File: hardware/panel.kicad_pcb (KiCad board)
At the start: 2 copper layers, 99.2 x 100 mm, 1073 parts, among them J1 USB_A_Embedded, U1 CH32V203F8U6, U2 XC6206PxxxMR

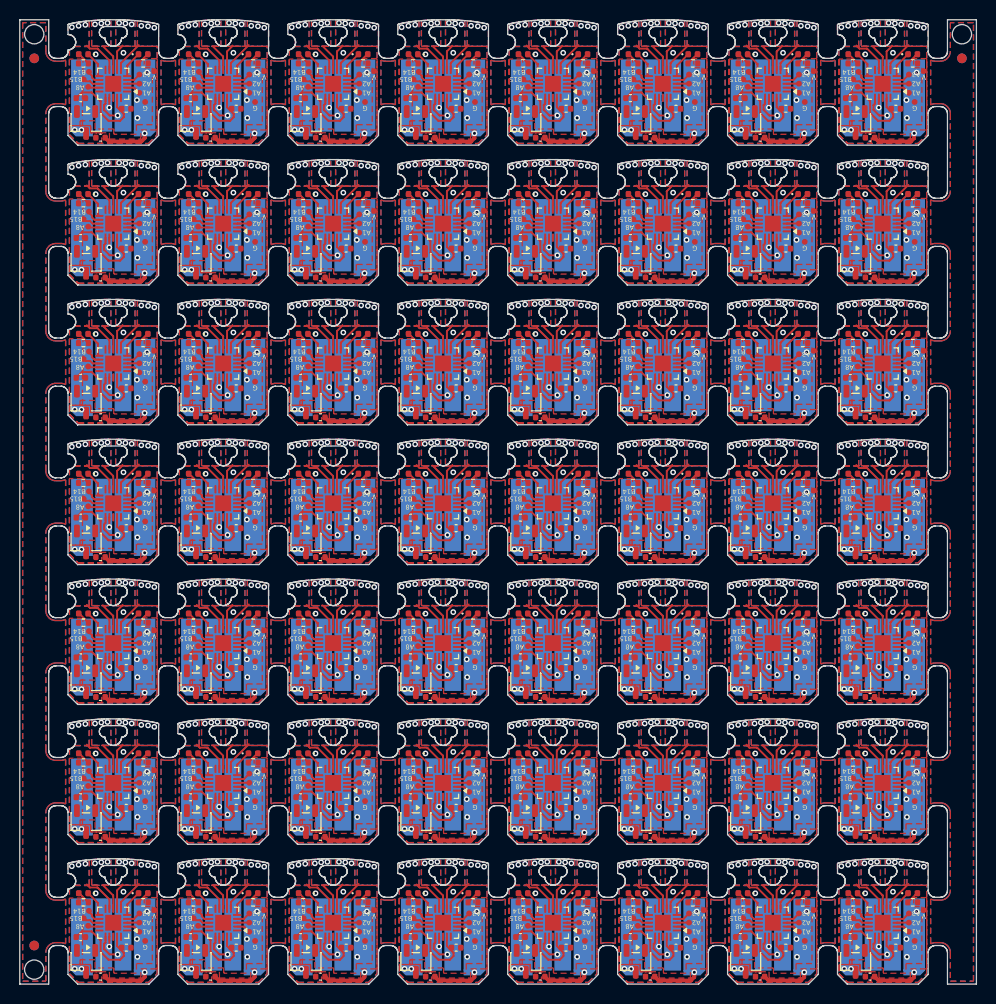
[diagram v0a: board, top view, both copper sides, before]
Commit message: Update
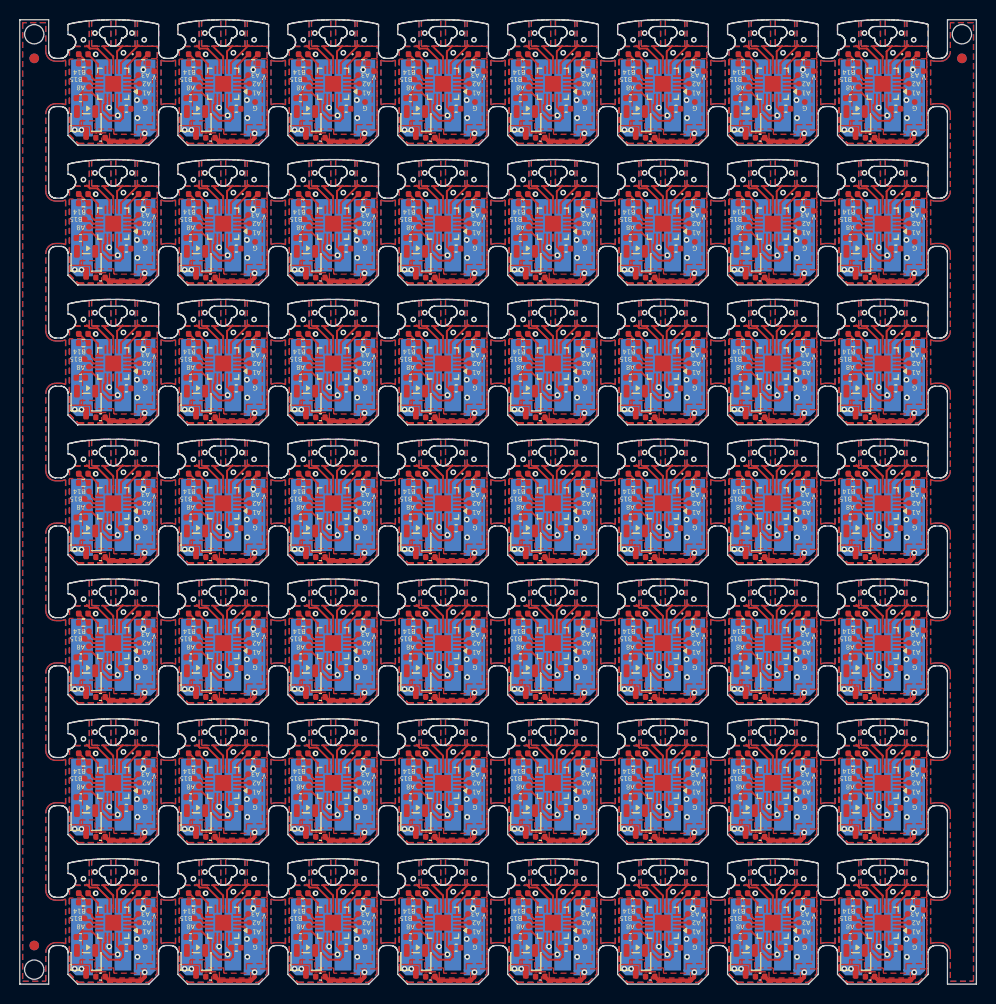
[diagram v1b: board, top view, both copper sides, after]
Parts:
- removed the TP1 at (145.5, 112.7)
- removed the TP1 at (134.1, 25.7)
- removed the TP1 at (156.9, 83.7)
- removed the TP1 at (168.3, 98.2)
- removed the TP1 at (156.9, 54.7)
- removed the TP1 at (122.7, 54.7)
- removed the TP1 at (145.5, 54.7)
- removed the TP1 at (111.3, 83.7)
- removed the TP1 at (122.7, 69.2)
- removed the TP1 at (122.7, 112.7)
- removed the TP1 at (145.5, 98.2)
- removed the TP1 at (156.9, 25.7)
- removed the TP1 at (122.7, 40.2)
- removed the TP1 at (145.5, 40.2)
- removed the TP1 at (111.3, 112.7)
- removed the TP1 at (179.7, 25.7)
- removed the TP1 at (191.1, 112.7)
- removed the TP1 at (179.7, 112.7)
- removed the TP1 at (191.1, 98.2)
- removed the TP1 at (168.3, 25.7)
- removed the TP1 at (134.1, 69.2)
- removed the TP1 at (111.3, 54.7)
- removed the TP1 at (111.3, 40.2)
- removed the TP1 at (145.5, 83.7)
- removed the TP1 at (111.3, 25.7)
- removed the TP1 at (134.1, 40.2)
- removed the TP1 at (111.3, 69.2)
- removed the TP1 at (145.5, 25.7)
- removed the TP1 at (134.1, 83.7)
- removed the TP1 at (156.9, 69.2)
- removed the TP1 at (168.3, 54.7)
- removed the TP1 at (168.3, 112.7)
- removed the TP1 at (122.7, 83.7)
- removed the TP1 at (179.7, 69.2)
- removed the TP1 at (168.3, 69.2)
- removed the TP1 at (134.1, 112.7)
- removed the TP1 at (191.1, 25.7)
- removed the TP1 at (156.9, 112.7)
- removed the TP1 at (111.3, 98.2)
- removed the TP1 at (145.5, 69.2)
- removed the TP1 at (179.7, 98.2)
- removed the TP1 at (179.7, 54.7)
- removed the TP1 at (191.1, 69.2)
- removed the TP1 at (156.9, 98.2)
- removed the TP1 at (156.9, 40.2)
- removed the TP1 at (134.1, 98.2)
- removed the TP1 at (191.1, 83.7)
- removed the TP1 at (134.1, 54.7)
- removed the TP1 at (168.3, 83.7)
- removed the TP1 at (122.7, 98.2)
- removed the TP1 at (122.7, 25.7)
- removed the TP1 at (179.7, 40.2)
- removed the TP1 at (168.3, 40.2)
- removed the TP1 at (179.7, 83.7)
- removed the TP1 at (191.1, 54.7)
- removed the TP1 at (191.1, 40.2)
- removed the TP5 at (185.3, 55.2)
- removed the TP5 at (105.5, 69.7)
- removed the TP5 at (151.1, 98.7)
- removed the TP5 at (185.3, 113.2)
- removed the TP5 at (139.7, 26.2)
- removed the TP5 at (173.9, 84.2)
- removed the TP5 at (173.9, 69.7)
- removed the TP5 at (128.3, 84.2)
- removed the TP5 at (139.7, 98.7)
- removed the TP5 at (105.5, 55.2)
- removed the TP5 at (185.3, 98.7)
- removed the TP5 at (185.3, 69.7)
- removed the TP5 at (116.9, 98.7)
- removed the TP5 at (162.5, 113.2)
- removed the TP5 at (151.1, 55.2)
- removed the TP5 at (128.3, 69.7)
- removed the TP5 at (151.1, 113.2)
- removed the TP5 at (185.3, 26.2)
- removed the TP5 at (139.7, 40.7)
- removed the TP5 at (116.9, 84.2)
- removed the TP5 at (162.5, 55.2)
- removed the TP5 at (128.3, 40.7)
- removed the TP5 at (173.9, 40.7)
- removed the TP5 at (139.7, 69.7)
- removed the TP5 at (128.3, 113.2)
- removed the TP5 at (105.5, 84.2)
- removed the TP5 at (116.9, 26.2)
- removed the TP5 at (139.7, 55.2)
- removed the TP5 at (105.5, 113.2)
- removed the TP5 at (151.1, 26.2)
- removed the TP5 at (139.7, 113.2)
- removed the TP5 at (105.5, 98.7)
- removed the TP5 at (162.5, 40.7)
- removed the TP5 at (128.3, 26.2)
- removed the TP5 at (173.9, 55.2)
- removed the TP5 at (116.9, 113.2)
- removed the TP5 at (173.9, 26.2)
- removed the TP5 at (105.5, 26.2)
- removed the TP5 at (185.3, 84.2)
- removed the TP5 at (185.3, 40.7)
- removed the TP5 at (162.5, 84.2)
- removed the TP5 at (162.5, 26.2)
- removed the TP5 at (173.9, 98.7)
- removed the TP5 at (105.5, 40.7)
- removed the TP5 at (151.1, 40.7)
- removed the TP5 at (116.9, 40.7)
- removed the TP5 at (151.1, 84.2)
- removed the TP5 at (173.9, 113.2)
- removed the TP5 at (116.9, 69.7)
- removed the TP5 at (151.1, 69.7)
- removed the TP5 at (162.5, 98.7)
- removed the TP5 at (128.3, 55.2)
- removed the TP5 at (128.3, 98.7)
- removed the TP5 at (139.7, 84.2)
- removed the TP5 at (162.5, 69.7)
- removed the TP5 at (116.9, 55.2)
- removed the TP6 at (106.0, 56.0)
- removed the TP6 at (140.2, 70.5)
- removed the TP6 at (140.2, 114.0)
- removed the TP6 at (106.0, 85.0)
- removed the TP6 at (140.2, 56.0)
- removed the TP6 at (151.6, 41.5)
- removed the TP6 at (117.4, 70.5)
- removed the TP6 at (117.4, 56.0)
- removed the TP6 at (106.0, 41.5)
- removed the TP6 at (163.0, 85.0)
- removed the TP6 at (106.0, 70.5)
- removed the TP6 at (163.0, 114.0)
- removed the TP6 at (117.4, 85.0)
- removed the TP6 at (185.8, 85.0)
- removed the TP6 at (185.8, 70.5)
- removed the TP6 at (151.6, 99.5)
- removed the TP6 at (185.8, 41.5)
- removed the TP6 at (140.2, 99.5)
- removed the TP6 at (185.8, 114.0)
- removed the TP6 at (163.0, 70.5)
- removed the TP6 at (174.4, 114.0)
- removed the TP6 at (128.8, 41.5)
- removed the TP6 at (106.0, 114.0)
- removed the TP6 at (151.6, 56.0)
- removed the TP6 at (174.4, 41.5)
- removed the TP6 at (174.4, 56.0)
- removed the TP6 at (140.2, 27.0)
- removed the TP6 at (174.4, 85.0)
- removed the TP6 at (128.8, 99.5)
- removed the TP6 at (117.4, 41.5)
- removed the TP6 at (151.6, 85.0)
- removed the TP6 at (163.0, 27.0)
- removed the TP6 at (128.8, 56.0)
- removed the TP6 at (117.4, 114.0)
- removed the TP6 at (185.8, 56.0)
- removed the TP6 at (151.6, 114.0)
- removed the TP6 at (117.4, 27.0)
- removed the TP6 at (128.8, 27.0)
- removed the TP6 at (117.4, 99.5)
- removed the TP6 at (128.8, 70.5)
- removed the TP6 at (106.0, 27.0)
- removed the TP6 at (128.8, 85.0)
- removed the TP6 at (163.0, 41.5)
- removed the TP6 at (106.0, 99.5)
- removed the TP6 at (174.4, 99.5)
- removed the TP6 at (163.0, 56.0)
- removed the TP6 at (151.6, 70.5)
- removed the TP6 at (163.0, 99.5)
- removed the TP6 at (151.6, 27.0)
- removed the TP6 at (128.8, 114.0)
- removed the TP6 at (185.8, 27.0)
- removed the TP6 at (174.4, 70.5)
- removed the TP6 at (140.2, 41.5)
- removed the TP6 at (140.2, 85.0)
- removed the TP6 at (174.4, 27.0)
- removed the TP6 at (185.8, 99.5)
- added TP1: TestPoint, ch32:TestPoint_Pad_D0.6mm, F.Cu at (168.2, 83.7)
- added TP1: TestPoint, ch32:TestPoint_Pad_D0.6mm, F.Cu at (156.8, 69.2)
- added TP1: TestPoint, ch32:TestPoint_Pad_D0.6mm, F.Cu at (145.4, 40.2)
- added TP1: TestPoint, ch32:TestPoint_Pad_D0.6mm, F.Cu at (179.6, 69.2)
- added TP1: TestPoint, ch32:TestPoint_Pad_D0.6mm, F.Cu at (179.6, 112.7)
- added TP1: TestPoint, ch32:TestPoint_Pad_D0.6mm, F.Cu at (111.2, 69.2)
- added TP1: TestPoint, ch32:TestPoint_Pad_D0.6mm, F.Cu at (111.2, 83.7)
- added TP1: TestPoint, ch32:TestPoint_Pad_D0.6mm, F.Cu at (179.6, 83.7)
- added TP1: TestPoint, ch32:TestPoint_Pad_D0.6mm, F.Cu at (122.6, 25.7)
- added TP1: TestPoint, ch32:TestPoint_Pad_D0.6mm, F.Cu at (156.8, 54.7)
- added TP1: TestPoint, ch32:TestPoint_Pad_D0.6mm, F.Cu at (134.0, 40.2)
- added TP1: TestPoint, ch32:TestPoint_Pad_D0.6mm, F.Cu at (168.2, 54.7)
- added TP1: TestPoint, ch32:TestPoint_Pad_D0.6mm, F.Cu at (134.0, 25.7)
- added TP1: TestPoint, ch32:TestPoint_Pad_D0.6mm, F.Cu at (156.8, 83.7)
- added TP1: TestPoint, ch32:TestPoint_Pad_D0.6mm, F.Cu at (156.8, 98.2)
- added TP1: TestPoint, ch32:TestPoint_Pad_D0.6mm, F.Cu at (191.0, 69.2)
- added TP1: TestPoint, ch32:TestPoint_Pad_D0.6mm, F.Cu at (134.0, 83.7)
- added TP1: TestPoint, ch32:TestPoint_Pad_D0.6mm, F.Cu at (134.0, 112.7)
- added TP1: TestPoint, ch32:TestPoint_Pad_D0.6mm, F.Cu at (111.2, 54.7)
- added TP1: TestPoint, ch32:TestPoint_Pad_D0.6mm, F.Cu at (145.4, 98.2)
- added TP1: TestPoint, ch32:TestPoint_Pad_D0.6mm, F.Cu at (134.0, 69.2)
- added TP1: TestPoint, ch32:TestPoint_Pad_D0.6mm, F.Cu at (168.2, 112.7)
- added TP1: TestPoint, ch32:TestPoint_Pad_D0.6mm, F.Cu at (111.2, 40.2)
- added TP1: TestPoint, ch32:TestPoint_Pad_D0.6mm, F.Cu at (179.6, 25.7)
- added TP1: TestPoint, ch32:TestPoint_Pad_D0.6mm, F.Cu at (145.4, 25.7)
- added TP1: TestPoint, ch32:TestPoint_Pad_D0.6mm, F.Cu at (134.0, 54.7)
- added TP1: TestPoint, ch32:TestPoint_Pad_D0.6mm, F.Cu at (111.2, 25.7)
- added TP1: TestPoint, ch32:TestPoint_Pad_D0.6mm, F.Cu at (191.0, 112.7)
- added TP1: TestPoint, ch32:TestPoint_Pad_D0.6mm, F.Cu at (191.0, 83.7)
- added TP1: TestPoint, ch32:TestPoint_Pad_D0.6mm, F.Cu at (191.0, 25.7)
- added TP1: TestPoint, ch32:TestPoint_Pad_D0.6mm, F.Cu at (122.6, 40.2)
- added TP1: TestPoint, ch32:TestPoint_Pad_D0.6mm, F.Cu at (111.2, 98.2)
- added TP1: TestPoint, ch32:TestPoint_Pad_D0.6mm, F.Cu at (122.6, 83.7)
- added TP1: TestPoint, ch32:TestPoint_Pad_D0.6mm, F.Cu at (168.2, 69.2)
- added TP1: TestPoint, ch32:TestPoint_Pad_D0.6mm, F.Cu at (145.4, 54.7)
- added TP1: TestPoint, ch32:TestPoint_Pad_D0.6mm, F.Cu at (145.4, 112.7)
- added TP1: TestPoint, ch32:TestPoint_Pad_D0.6mm, F.Cu at (191.0, 98.2)
- added TP1: TestPoint, ch32:TestPoint_Pad_D0.6mm, F.Cu at (179.6, 40.2)
- added TP1: TestPoint, ch32:TestPoint_Pad_D0.6mm, F.Cu at (168.2, 25.7)
- added TP1: TestPoint, ch32:TestPoint_Pad_D0.6mm, F.Cu at (122.6, 54.7)
- added TP1: TestPoint, ch32:TestPoint_Pad_D0.6mm, F.Cu at (145.4, 83.7)
- added TP1: TestPoint, ch32:TestPoint_Pad_D0.6mm, F.Cu at (122.6, 98.2)
- added TP1: TestPoint, ch32:TestPoint_Pad_D0.6mm, F.Cu at (156.8, 40.2)
- added TP1: TestPoint, ch32:TestPoint_Pad_D0.6mm, F.Cu at (156.8, 112.7)
- added TP1: TestPoint, ch32:TestPoint_Pad_D0.6mm, F.Cu at (168.2, 98.2)
- added TP1: TestPoint, ch32:TestPoint_Pad_D0.6mm, F.Cu at (179.6, 98.2)
- added TP1: TestPoint, ch32:TestPoint_Pad_D0.6mm, F.Cu at (111.2, 112.7)
- added TP1: TestPoint, ch32:TestPoint_Pad_D0.6mm, F.Cu at (122.6, 69.2)
- added TP1: TestPoint, ch32:TestPoint_Pad_D0.6mm, F.Cu at (168.2, 40.2)
- added TP1: TestPoint, ch32:TestPoint_Pad_D0.6mm, F.Cu at (191.0, 54.7)
- added TP1: TestPoint, ch32:TestPoint_Pad_D0.6mm, F.Cu at (134.0, 98.2)
- added TP1: TestPoint, ch32:TestPoint_Pad_D0.6mm, F.Cu at (145.4, 69.2)
- added TP1: TestPoint, ch32:TestPoint_Pad_D0.6mm, F.Cu at (191.0, 40.2)
- added TP1: TestPoint, ch32:TestPoint_Pad_D0.6mm, F.Cu at (122.6, 112.7)
- added TP1: TestPoint, ch32:TestPoint_Pad_D0.6mm, F.Cu at (179.6, 54.7)
- added TP1: TestPoint, ch32:TestPoint_Pad_D0.6mm, F.Cu at (156.8, 25.7)
- added TP5: TestPoint, ch32:TestPoint_Pad_D0.6mm, F.Cu at (105.6, 69.7)
- added TP5: TestPoint, ch32:TestPoint_Pad_D0.6mm, F.Cu at (117.0, 69.7)
- added TP5: TestPoint, ch32:TestPoint_Pad_D0.6mm, F.Cu at (174.0, 113.2)
- added TP5: TestPoint, ch32:TestPoint_Pad_D0.6mm, F.Cu at (151.2, 40.7)
- added TP5: TestPoint, ch32:TestPoint_Pad_D0.6mm, F.Cu at (174.0, 98.7)
- added TP5: TestPoint, ch32:TestPoint_Pad_D0.6mm, F.Cu at (162.6, 40.7)
- added TP5: TestPoint, ch32:TestPoint_Pad_D0.6mm, F.Cu at (151.2, 98.7)
- added TP5: TestPoint, ch32:TestPoint_Pad_D0.6mm, F.Cu at (151.2, 69.7)
- added TP5: TestPoint, ch32:TestPoint_Pad_D0.6mm, F.Cu at (185.4, 113.2)
- added TP5: TestPoint, ch32:TestPoint_Pad_D0.6mm, F.Cu at (117.0, 84.2)
- added TP5: TestPoint, ch32:TestPoint_Pad_D0.6mm, F.Cu at (139.8, 26.2)
- added TP5: TestPoint, ch32:TestPoint_Pad_D0.6mm, F.Cu at (139.8, 69.7)
- added TP5: TestPoint, ch32:TestPoint_Pad_D0.6mm, F.Cu at (128.4, 69.7)
- added TP5: TestPoint, ch32:TestPoint_Pad_D0.6mm, F.Cu at (105.6, 98.7)
- added TP5: TestPoint, ch32:TestPoint_Pad_D0.6mm, F.Cu at (162.6, 69.7)
- added TP5: TestPoint, ch32:TestPoint_Pad_D0.6mm, F.Cu at (117.0, 98.7)
- added TP5: TestPoint, ch32:TestPoint_Pad_D0.6mm, F.Cu at (105.6, 113.2)
- added TP5: TestPoint, ch32:TestPoint_Pad_D0.6mm, F.Cu at (174.0, 26.2)
- added TP5: TestPoint, ch32:TestPoint_Pad_D0.6mm, F.Cu at (139.8, 84.2)
- added TP5: TestPoint, ch32:TestPoint_Pad_D0.6mm, F.Cu at (185.4, 55.2)
- added TP5: TestPoint, ch32:TestPoint_Pad_D0.6mm, F.Cu at (128.4, 113.2)
- added TP5: TestPoint, ch32:TestPoint_Pad_D0.6mm, F.Cu at (128.4, 55.2)
- added TP5: TestPoint, ch32:TestPoint_Pad_D0.6mm, F.Cu at (151.2, 84.2)
- added TP5: TestPoint, ch32:TestPoint_Pad_D0.6mm, F.Cu at (185.4, 84.2)
- added TP5: TestPoint, ch32:TestPoint_Pad_D0.6mm, F.Cu at (139.8, 55.2)
- added TP5: TestPoint, ch32:TestPoint_Pad_D0.6mm, F.Cu at (128.4, 84.2)
- added TP5: TestPoint, ch32:TestPoint_Pad_D0.6mm, F.Cu at (105.6, 84.2)
- added TP5: TestPoint, ch32:TestPoint_Pad_D0.6mm, F.Cu at (117.0, 26.2)
- added TP5: TestPoint, ch32:TestPoint_Pad_D0.6mm, F.Cu at (162.6, 98.7)
- added TP5: TestPoint, ch32:TestPoint_Pad_D0.6mm, F.Cu at (185.4, 69.7)
- added TP5: TestPoint, ch32:TestPoint_Pad_D0.6mm, F.Cu at (117.0, 40.7)
- added TP5: TestPoint, ch32:TestPoint_Pad_D0.6mm, F.Cu at (105.6, 55.2)
- added TP5: TestPoint, ch32:TestPoint_Pad_D0.6mm, F.Cu at (185.4, 26.2)
- added TP5: TestPoint, ch32:TestPoint_Pad_D0.6mm, F.Cu at (151.2, 55.2)
- added TP5: TestPoint, ch32:TestPoint_Pad_D0.6mm, F.Cu at (174.0, 69.7)
- added TP5: TestPoint, ch32:TestPoint_Pad_D0.6mm, F.Cu at (151.2, 113.2)
- added TP5: TestPoint, ch32:TestPoint_Pad_D0.6mm, F.Cu at (128.4, 98.7)
- added TP5: TestPoint, ch32:TestPoint_Pad_D0.6mm, F.Cu at (162.6, 84.2)
- added TP5: TestPoint, ch32:TestPoint_Pad_D0.6mm, F.Cu at (162.6, 26.2)
- added TP5: TestPoint, ch32:TestPoint_Pad_D0.6mm, F.Cu at (174.0, 40.7)
- added TP5: TestPoint, ch32:TestPoint_Pad_D0.6mm, F.Cu at (128.4, 26.2)
- added TP5: TestPoint, ch32:TestPoint_Pad_D0.6mm, F.Cu at (185.4, 98.7)
- added TP5: TestPoint, ch32:TestPoint_Pad_D0.6mm, F.Cu at (162.6, 55.2)
- added TP5: TestPoint, ch32:TestPoint_Pad_D0.6mm, F.Cu at (162.6, 113.2)
- added TP5: TestPoint, ch32:TestPoint_Pad_D0.6mm, F.Cu at (105.6, 26.2)
- added TP5: TestPoint, ch32:TestPoint_Pad_D0.6mm, F.Cu at (139.8, 40.7)
- added TP5: TestPoint, ch32:TestPoint_Pad_D0.6mm, F.Cu at (117.0, 113.2)
- added TP5: TestPoint, ch32:TestPoint_Pad_D0.6mm, F.Cu at (139.8, 98.7)
- added TP5: TestPoint, ch32:TestPoint_Pad_D0.6mm, F.Cu at (185.4, 40.7)
- added TP5: TestPoint, ch32:TestPoint_Pad_D0.6mm, F.Cu at (117.0, 55.2)
- added TP5: TestPoint, ch32:TestPoint_Pad_D0.6mm, F.Cu at (139.8, 113.2)
- added TP5: TestPoint, ch32:TestPoint_Pad_D0.6mm, F.Cu at (174.0, 55.2)
- added TP5: TestPoint, ch32:TestPoint_Pad_D0.6mm, F.Cu at (174.0, 84.2)
- added TP5: TestPoint, ch32:TestPoint_Pad_D0.6mm, F.Cu at (128.4, 40.7)
- added TP5: TestPoint, ch32:TestPoint_Pad_D0.6mm, F.Cu at (151.2, 26.2)
- added TP5: TestPoint, ch32:TestPoint_Pad_D0.6mm, F.Cu at (105.6, 40.7)
- added TP6: TestPoint, ch32:TestPoint_Pad_D0.6mm, F.Cu at (140.3, 114.0)
- added TP6: TestPoint, ch32:TestPoint_Pad_D0.6mm, F.Cu at (151.7, 70.5)
- added TP6: TestPoint, ch32:TestPoint_Pad_D0.6mm, F.Cu at (185.9, 27.0)
- added TP6: TestPoint, ch32:TestPoint_Pad_D0.6mm, F.Cu at (128.9, 85.0)
- added TP6: TestPoint, ch32:TestPoint_Pad_D0.6mm, F.Cu at (117.5, 41.5)
- added TP6: TestPoint, ch32:TestPoint_Pad_D0.6mm, F.Cu at (185.9, 114.0)
- added TP6: TestPoint, ch32:TestPoint_Pad_D0.6mm, F.Cu at (163.1, 27.0)
- added TP6: TestPoint, ch32:TestPoint_Pad_D0.6mm, F.Cu at (151.7, 41.5)
- added TP6: TestPoint, ch32:TestPoint_Pad_D0.6mm, F.Cu at (174.5, 85.0)
- added TP6: TestPoint, ch32:TestPoint_Pad_D0.6mm, F.Cu at (106.1, 85.0)
- added TP6: TestPoint, ch32:TestPoint_Pad_D0.6mm, F.Cu at (151.7, 27.0)
- added TP6: TestPoint, ch32:TestPoint_Pad_D0.6mm, F.Cu at (163.1, 85.0)
- added TP6: TestPoint, ch32:TestPoint_Pad_D0.6mm, F.Cu at (163.1, 56.0)
- added TP6: TestPoint, ch32:TestPoint_Pad_D0.6mm, F.Cu at (151.7, 114.0)
- added TP6: TestPoint, ch32:TestPoint_Pad_D0.6mm, F.Cu at (140.3, 70.5)
- added TP6: TestPoint, ch32:TestPoint_Pad_D0.6mm, F.Cu at (128.9, 41.5)
- added TP6: TestPoint, ch32:TestPoint_Pad_D0.6mm, F.Cu at (106.1, 70.5)
- added TP6: TestPoint, ch32:TestPoint_Pad_D0.6mm, F.Cu at (174.5, 114.0)
- added TP6: TestPoint, ch32:TestPoint_Pad_D0.6mm, F.Cu at (185.9, 85.0)
- added TP6: TestPoint, ch32:TestPoint_Pad_D0.6mm, F.Cu at (163.1, 99.5)
- added TP6: TestPoint, ch32:TestPoint_Pad_D0.6mm, F.Cu at (174.5, 99.5)
- added TP6: TestPoint, ch32:TestPoint_Pad_D0.6mm, F.Cu at (185.9, 56.0)
- added TP6: TestPoint, ch32:TestPoint_Pad_D0.6mm, F.Cu at (151.7, 56.0)
- added TP6: TestPoint, ch32:TestPoint_Pad_D0.6mm, F.Cu at (128.9, 56.0)
- added TP6: TestPoint, ch32:TestPoint_Pad_D0.6mm, F.Cu at (117.5, 114.0)
- added TP6: TestPoint, ch32:TestPoint_Pad_D0.6mm, F.Cu at (128.9, 70.5)
- added TP6: TestPoint, ch32:TestPoint_Pad_D0.6mm, F.Cu at (185.9, 41.5)
- added TP6: TestPoint, ch32:TestPoint_Pad_D0.6mm, F.Cu at (151.7, 85.0)
- added TP6: TestPoint, ch32:TestPoint_Pad_D0.6mm, F.Cu at (128.9, 27.0)
- added TP6: TestPoint, ch32:TestPoint_Pad_D0.6mm, F.Cu at (163.1, 114.0)
- added TP6: TestPoint, ch32:TestPoint_Pad_D0.6mm, F.Cu at (174.5, 41.5)
- added TP6: TestPoint, ch32:TestPoint_Pad_D0.6mm, F.Cu at (117.5, 85.0)
- added TP6: TestPoint, ch32:TestPoint_Pad_D0.6mm, F.Cu at (140.3, 41.5)
- added TP6: TestPoint, ch32:TestPoint_Pad_D0.6mm, F.Cu at (151.7, 99.5)
- added TP6: TestPoint, ch32:TestPoint_Pad_D0.6mm, F.Cu at (117.5, 56.0)
- added TP6: TestPoint, ch32:TestPoint_Pad_D0.6mm, F.Cu at (106.1, 56.0)
- added TP6: TestPoint, ch32:TestPoint_Pad_D0.6mm, F.Cu at (128.9, 114.0)
- added TP6: TestPoint, ch32:TestPoint_Pad_D0.6mm, F.Cu at (117.5, 70.5)
- added TP6: TestPoint, ch32:TestPoint_Pad_D0.6mm, F.Cu at (174.5, 56.0)
- added TP6: TestPoint, ch32:TestPoint_Pad_D0.6mm, F.Cu at (140.3, 85.0)
- added TP6: TestPoint, ch32:TestPoint_Pad_D0.6mm, F.Cu at (163.1, 41.5)
- added TP6: TestPoint, ch32:TestPoint_Pad_D0.6mm, F.Cu at (106.1, 99.5)
- added TP6: TestPoint, ch32:TestPoint_Pad_D0.6mm, F.Cu at (106.1, 114.0)
- added TP6: TestPoint, ch32:TestPoint_Pad_D0.6mm, F.Cu at (185.9, 99.5)
- added TP6: TestPoint, ch32:TestPoint_Pad_D0.6mm, F.Cu at (174.5, 70.5)
- added TP6: TestPoint, ch32:TestPoint_Pad_D0.6mm, F.Cu at (128.9, 99.5)
- added TP6: TestPoint, ch32:TestPoint_Pad_D0.6mm, F.Cu at (117.5, 99.5)
- added TP6: TestPoint, ch32:TestPoint_Pad_D0.6mm, F.Cu at (106.1, 27.0)
- added TP6: TestPoint, ch32:TestPoint_Pad_D0.6mm, F.Cu at (106.1, 41.5)
- added TP6: TestPoint, ch32:TestPoint_Pad_D0.6mm, F.Cu at (140.3, 27.0)
- added TP6: TestPoint, ch32:TestPoint_Pad_D0.6mm, F.Cu at (140.3, 56.0)
- added TP6: TestPoint, ch32:TestPoint_Pad_D0.6mm, F.Cu at (185.9, 70.5)
- added TP6: TestPoint, ch32:TestPoint_Pad_D0.6mm, F.Cu at (140.3, 99.5)
- added TP6: TestPoint, ch32:TestPoint_Pad_D0.6mm, F.Cu at (163.1, 70.5)
- added TP6: TestPoint, ch32:TestPoint_Pad_D0.6mm, F.Cu at (174.5, 27.0)
- added TP6: TestPoint, ch32:TestPoint_Pad_D0.6mm, F.Cu at (117.5, 27.0)
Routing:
- net Board_5-/CAP1A: vias 3 -> 1
- net Board_4-/CAP1A: vias 3 -> 1
- net Board_3-/CAP1A: vias 3 -> 1
- net Board_1-/CAP1A: vias 3 -> 1
- net Board_0-/CAP1A: vias 3 -> 1
- net Board_9-/CAP1B: vias 3 -> 1
- net Board_9-/CAP1A: vias 3 -> 1
- net Board_9-/CAP0B: vias 3 -> 1
- net Board_9-/CAP0A: vias 3 -> 1
- net Board_8-/CAP1B: vias 3 -> 1
- net Board_8-/CAP1A: vias 3 -> 1
- net Board_8-/CAP0B: vias 3 -> 1
- net Board_8-/CAP0A: vias 3 -> 1
- net Board_7-/CAP1B: vias 3 -> 1
- net Board_7-/CAP1A: vias 3 -> 1
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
